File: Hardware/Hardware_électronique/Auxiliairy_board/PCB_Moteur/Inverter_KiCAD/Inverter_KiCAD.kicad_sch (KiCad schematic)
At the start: 17 parts, among them J1 Conn_02x02_Top_Bottom, J101 Conn_01x02, J2 Conn_02x03_Top_Bottom

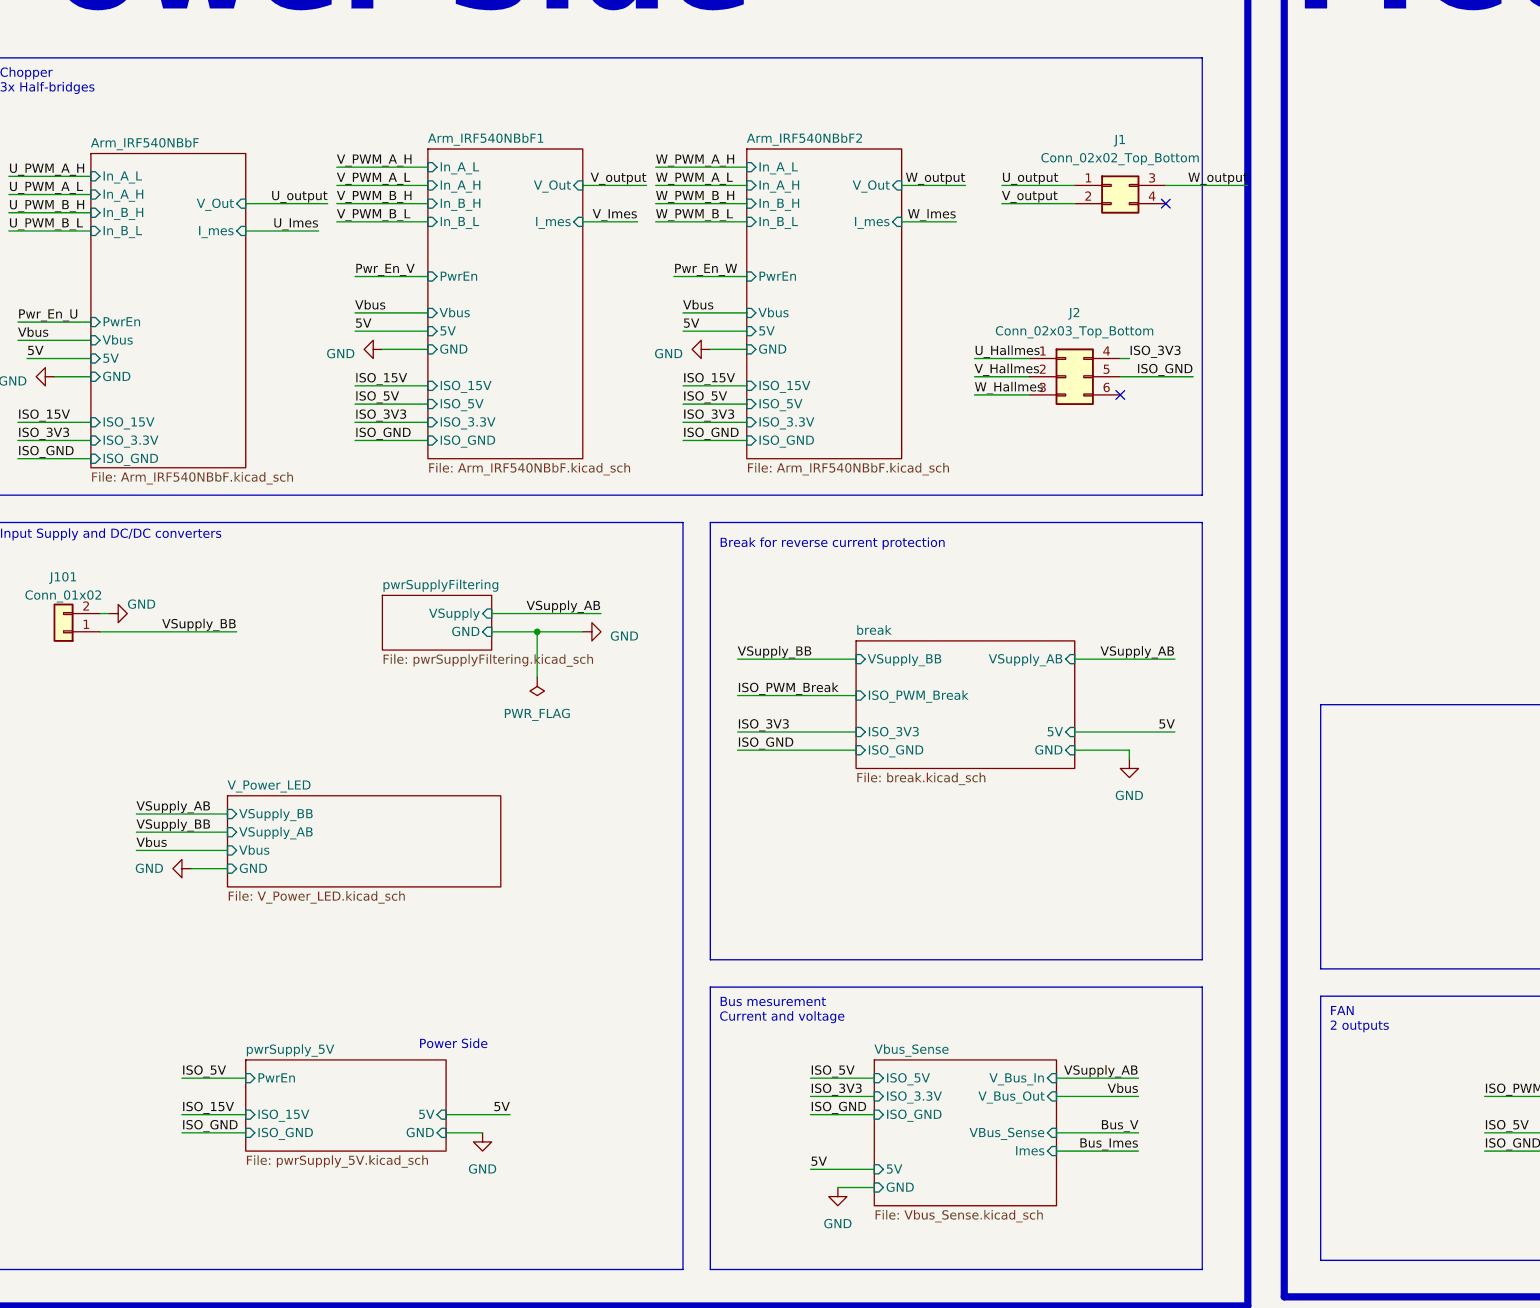
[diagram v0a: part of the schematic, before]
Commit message: Add files via upload
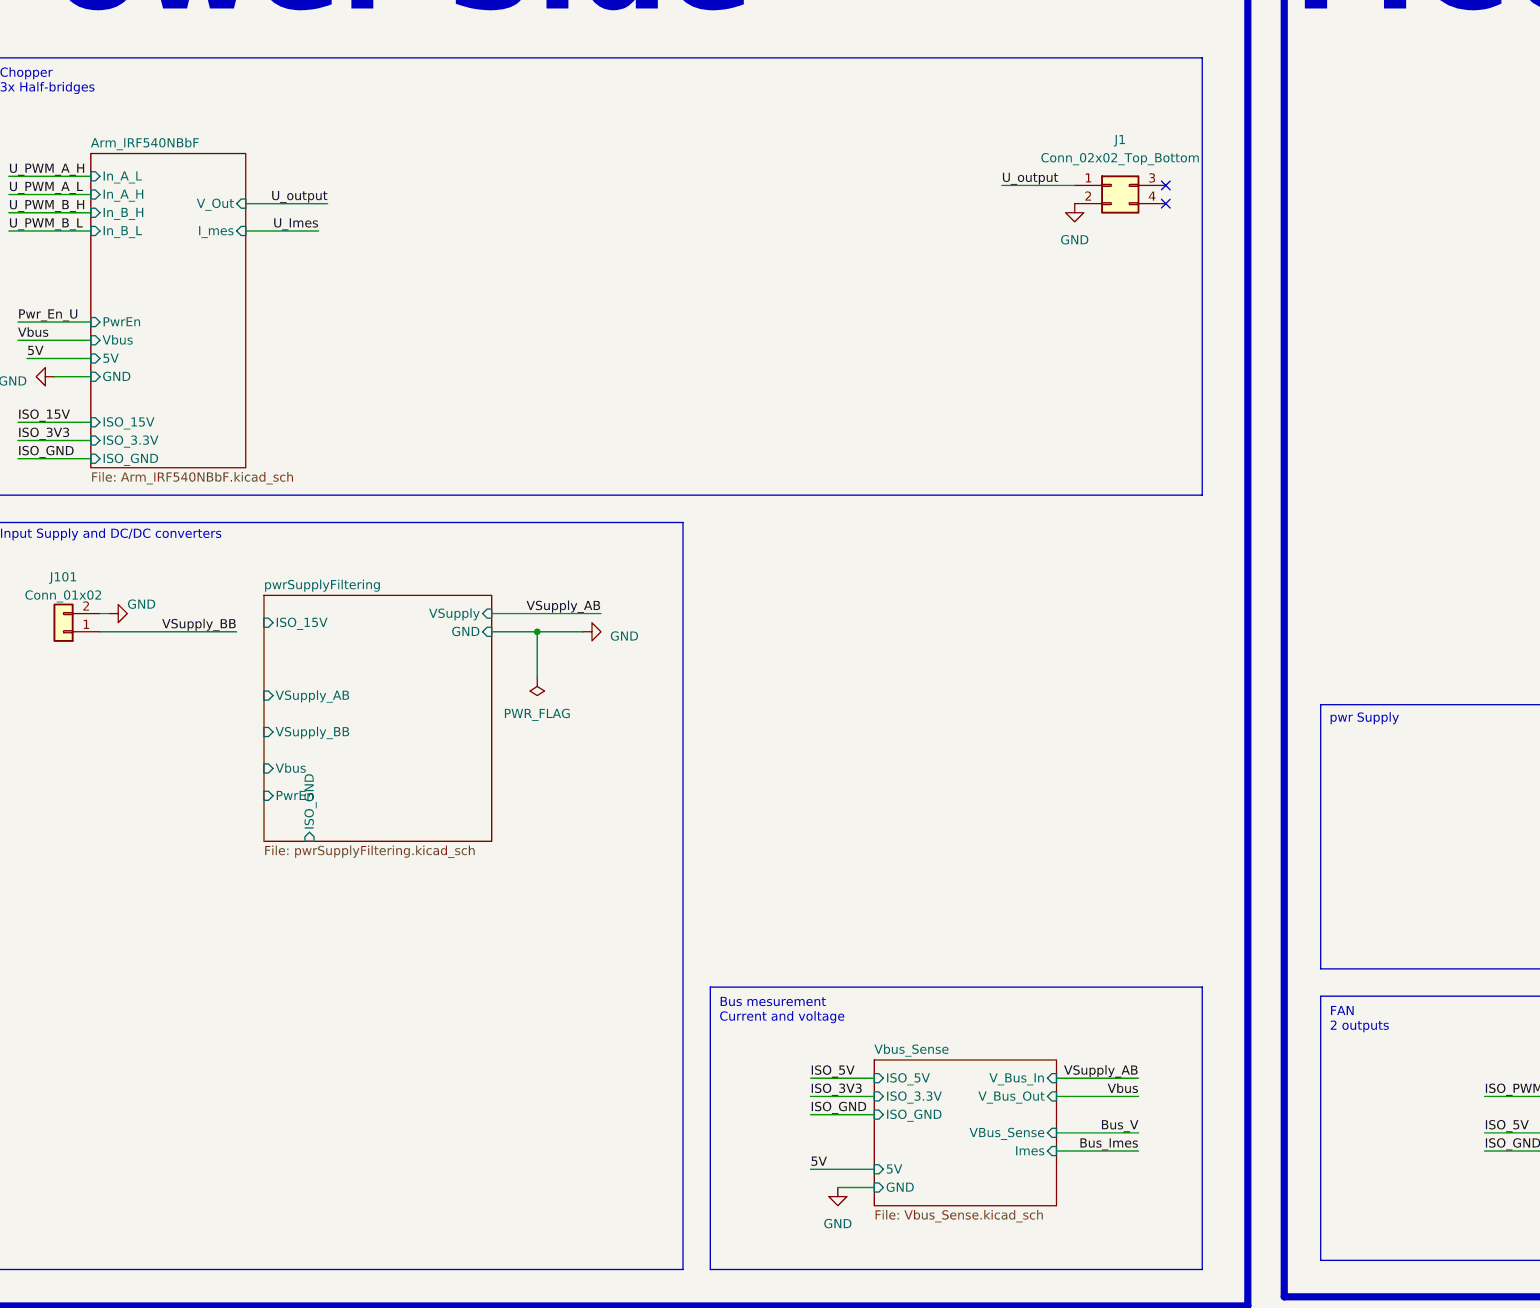
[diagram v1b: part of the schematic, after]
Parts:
- removed J2: Conn_02x03_Top_Bottom, Connector_Molex:Molex_Mega-Fit_76825-0006_2x03_P5.70mm_Horizontal, symbol Connector_Generic:Conn_02x03_Top_Bottom
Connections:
- net V_output is gone; now on net GND: J1.2 (Pin_2)
- net W_output: no longer names the net of J1.3 (Pin_3)
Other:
- removed sheet Arm_IRF540NBbF1
- removed sheet Arm_IRF540NBbF2
- removed sheet V_Power_LED
- removed sheet break
- removed sheet pwrSupply_5V
- sheet pwrSupplyFiltering ports: added ISO_15V, ISO_GND, PwrEn, VSupply_AB, VSupply_BB, Vbus; removed none
- note added: "pwr Supply"
- note removed: "Break for reverse current protection"
